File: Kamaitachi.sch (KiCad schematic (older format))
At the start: 88 parts, among them SW1 SW_PUSH, SW10 SW_PUSH, SW11 SW_PUSH, SW12 SW_PUSH, SW13 SW_PUSH, SW14 SW_PUSH, SW15 SW_PUSH, SW16 SW_PUSH, SW17 SW_PUSH, SW18 SW_PUSH, SW19 SW_PUSH, SW2 SW_PUSH, SW20 SW_PUSH, SW21 SW_PUSH, SW22 SW_PUSH, SW23 SW_PUSH, SW24 SW_PUSH, SW25 SW_PUSH, SW26 SW_PUSH, SW27 SW_PUSH, SW28 SW_PUSH, SW29 SW_PUSH, SW3 SW_PUSH, SW30 SW_PUSH, SW31 SW_PUSH, SW32 SW_PUSH, SW33 SW_PUSH, SW34 SW_PUSH, SW35 SW_PUSH, SW36 SW_PUSH, SW37 SW_PUSH, SW38 SW_PUSH, SW39 SW_PUSH, SW4 SW_PUSH, SW40 SW_PUSH, SW41 SW_PUSH, SW42 SW_PUSH, SW43 SW_PUSH, SW44 SW_PUSH, SW5 SW_PUSH, SW6 SW_PUSH, SW7 SW_PUSH, SW8 SW_PUSH, SW9 SW_PUSH, U1 ProMicro

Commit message: pcb in progress
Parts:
- SW1, SW10, SW11, SW12, SW13, SW14, SW15, SW16, SW17, SW19, SW2, SW20, SW21, SW22, SW23, SW24, SW25, SW27, SW28, SW29, SW3, SW30, SW31, SW32, SW33, SW34, SW35, SW36, SW37, SW38, SW39, SW4, SW41, SW42, SW43, SW5, SW6, SW8, SW9: footprint Keebio-Parts:MX_PCB_100H -> emptystring:CherryMX_Hotswap_Back
- SW18, SW26: footprint Keebio-Parts:MX_PCB_125H -> emptystring:CherryMX_Hotswap_Back
- SW40, SW7: footprint Keebio-Parts:MX_PCB_150H -> emptystring:CherryMX_Hotswap_Back
- SW44: footprint Keebio-Parts:MX_PCB_100H -> kbd:ResetSW
- U1: symbol kbd:ProMicro -> Kamaitachi-rescue:ProMicro-kbd

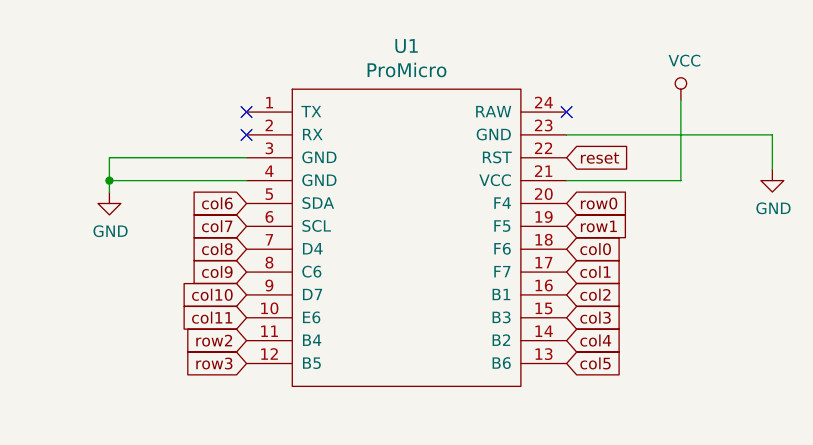
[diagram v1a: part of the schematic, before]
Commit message: pcb finished
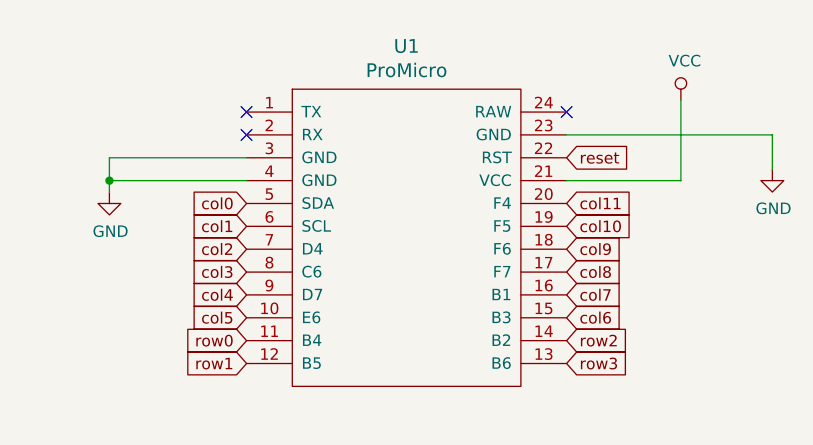
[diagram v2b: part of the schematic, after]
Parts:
- SW1, SW10, SW11, SW12, SW13, SW14, SW15, SW16, SW17, SW19, SW2, SW20, SW21, SW22, SW23, SW24, SW25, SW27, SW28, SW29, SW3, SW30, SW31, SW32, SW33, SW34, SW35, SW36, SW37, SW38, SW39, SW4, SW41, SW42, SW43, SW5, SW6, SW8, SW9: footprint emptystring:CherryMX_Hotswap_Back -> Keebio-Parts:MX_PCB_100H
- SW18, SW26: footprint emptystring:CherryMX_Hotswap_Back -> Keebio-Parts:MX_PCB_125H
- SW40, SW7: footprint emptystring:CherryMX_Hotswap_Back -> Keebio-Parts:MX_PCB_150H
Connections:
- net col0: now also U1.5 (SDA); no longer U1.18 (F6)
- net col1: now also U1.6 (SCL); no longer U1.17 (F7)
- net col10: now also U1.19 (F5); no longer U1.9 (D7)
- net col11: now also U1.20 (F4); no longer U1.10 (E6)
- net col2: now also U1.7 (D4); no longer U1.16 (B1)
- net col3: now also U1.8 (C6); no longer U1.15 (B3)
- net col4: now also U1.9 (D7); no longer U1.14 (B2)
- net col5: now also U1.10 (E6); no longer U1.13 (B6)
- net col6: now also U1.15 (B3); no longer U1.5 (SDA)
- net col7: now also U1.16 (B1); no longer U1.6 (SCL)
- net col8: now also U1.17 (F7); no longer U1.7 (D4)
- net col9: now also U1.18 (F6); no longer U1.8 (C6)
- net row0: now also U1.11 (B4); no longer U1.20 (F4)
- net row1: now also U1.12 (B5); no longer U1.19 (F5)
- net row2: now also U1.14 (B2); no longer U1.11 (B4)
- net row3: now also U1.13 (B6); no longer U1.12 (B5)
